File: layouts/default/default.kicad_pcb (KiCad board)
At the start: 2 copper layers, 41.9 x 35.3 mm, 43 parts

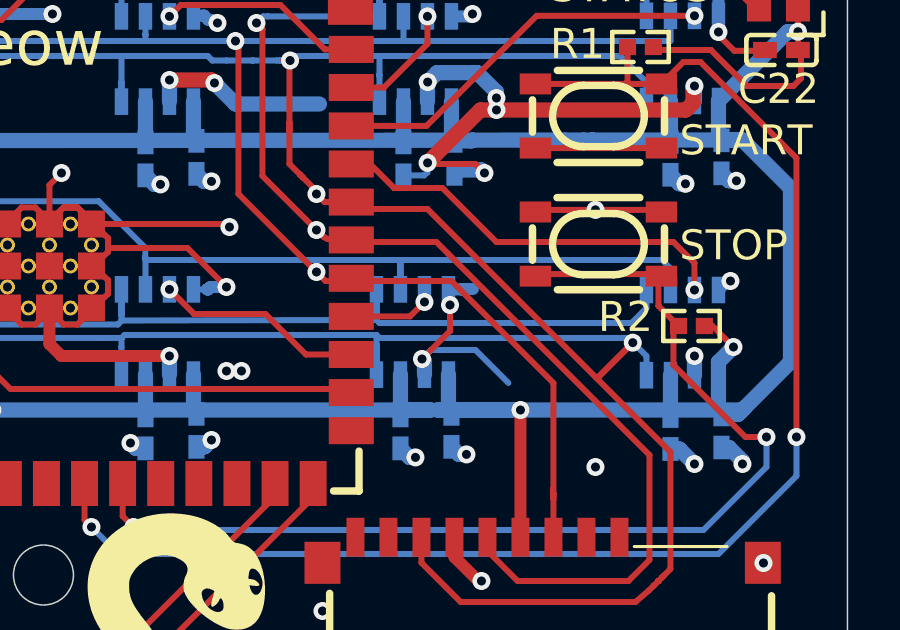
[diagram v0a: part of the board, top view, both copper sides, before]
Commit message: ordered
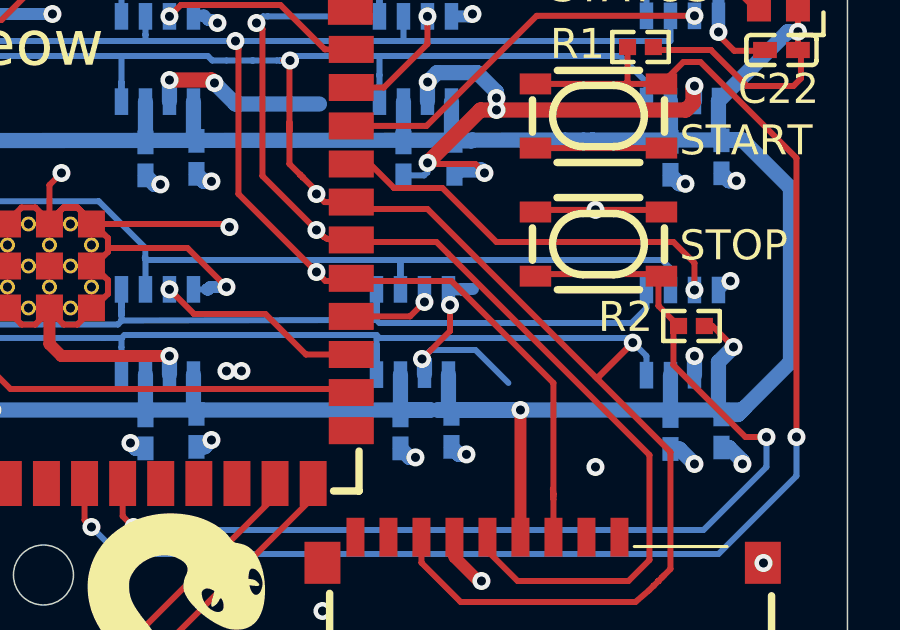
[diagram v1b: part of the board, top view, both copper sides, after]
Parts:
- C1, C2: value 10µF ±10% 25V X5R -> 100nF ±10% 50V X7R
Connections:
- net SUB1 renamed A8
- R1 pad 2: input-2 -> input
- R6 pad 2: input -> input-2
- U10 pad 2: CSB-4 -> CSB-5
- U11 pad 2: line-2 -> line
- U12 pad 2: CSB-5 -> CSB
- U13 pad 2: CSB -> CSB-1
- U15 pad 1: input-2 -> input
- U15 pad 2: input-2 -> input
- U2 pad 2: CSB-2 -> CSB-4
- U3 pad 2: CSB-1 -> CSB-2
- U4 pad 16: CSB -> CSB-1
- U4 pad 17: CSB-5 -> CSB
- U4 pad 18: line-2 -> line
- U4 pad 22: CSB-4 -> CSB-5
- U4 pad 25: CSB-1 -> CSB-2
- U4 pad 26: CSB-2 -> CSB-4
- U4 pad 8: line -> line-1
- U4 pad 9: line-1 -> line-2
- U7 pad 1: input -> input-2
- U7 pad 2: input -> input-2
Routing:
- net input-2: track 48.6 -> 17.9 mm
- net input: track 17.9 -> 48.6 mm
- net CSB-1: track 6.83 -> 15.7 mm
- net CSB: track 15.7 -> 6.96 mm
- net CSB-2: track 14.3 -> 6.83 mm
- net CSB-5: track 6.96 -> 13.7 mm
- net line-2: track 2.64 -> 0.00 mm, vias 1 -> 0
- net line: track 0.00 -> 2.64 mm, vias 0 -> 1
- net CSB-4: track 13.7 -> 14.3 mm
